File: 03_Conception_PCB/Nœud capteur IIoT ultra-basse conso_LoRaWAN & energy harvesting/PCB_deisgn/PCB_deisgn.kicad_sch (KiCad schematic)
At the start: 24 parts, among them J1 SWD1, U1 AEM10941-QFN, U2 STM32U073C8Ux, Y1 Crystal

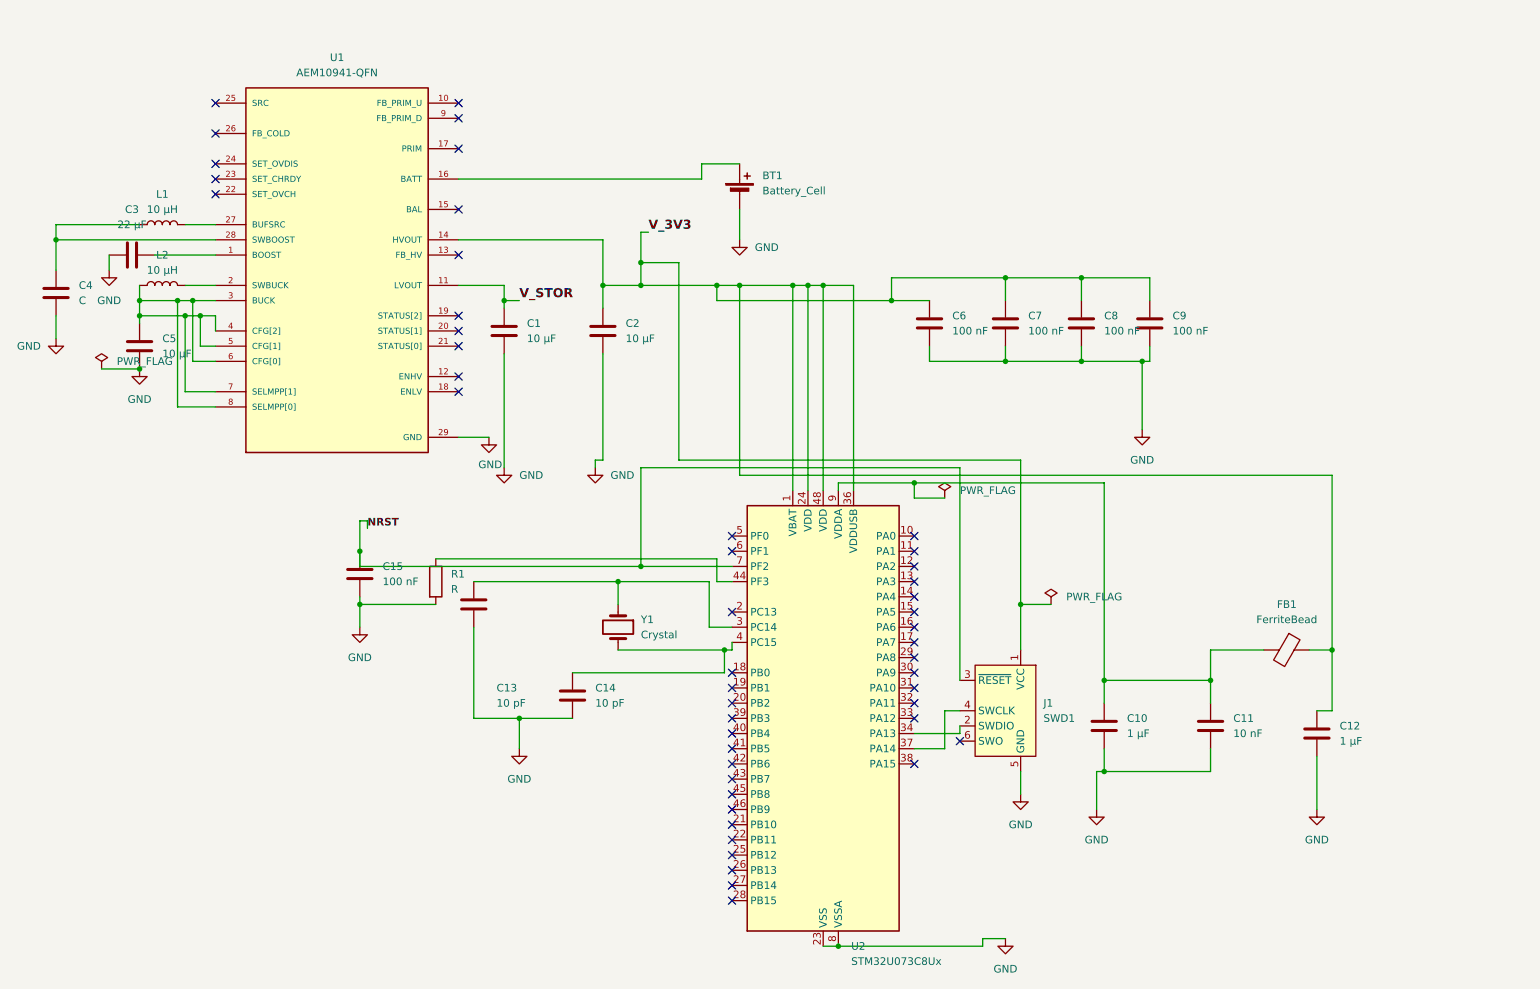
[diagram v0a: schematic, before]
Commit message: UPDATE
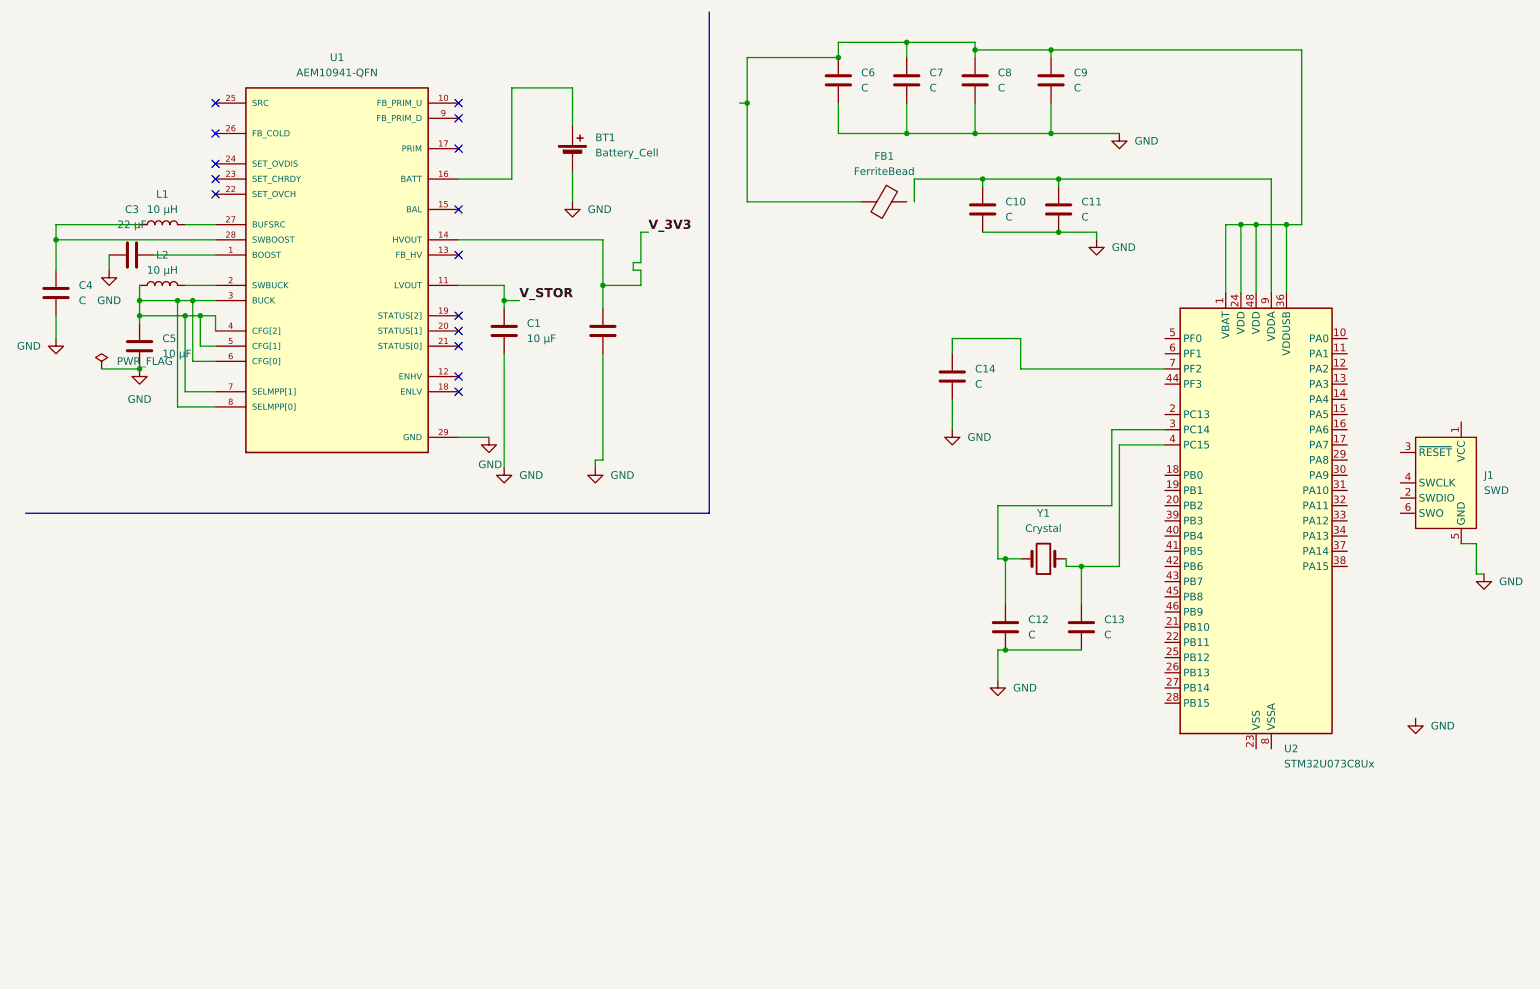
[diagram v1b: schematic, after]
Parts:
- removed C15: 100 nF, symbol Device:C
- removed R1: R, symbol Device:R
- C10, C12: value 1 µF -> C
- C11: value 10 nF -> C
- C13, C14: value 10 pF -> C
- C6, C7, C8, C9: value 100 nF -> C
- FB1: footprint (none) -> Inductor_SMD:L_6.3x6.3_H3
- J1: value SWD1 -> SWD
- Y1: footprint Crystal:Crystal_AT310_D3.0mm_L10.0mm_Horizontal -> (none)
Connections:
- net GND: no longer U2.23 (VSS), U2.35 (VSS), U2.47 (VSS), U2.49 (VSS), U2.8 (VSSA)
- net V_3V3: no longer C12.1, C6.1, C7.1, C8.1, C9.1, FB1.1, J1.1 (VCC), U2.1 (VBAT), U2.24 (VDD), U2.36 (VDDUSB), U2.48 (VDD)
- net at C10.1, C11.1, U2.9 (VDDA): no longer FB1.2
- net at J1.2 (SWDIO): no longer U2.34 (PA13)
- net at J1.4 (SWCLK): no longer U2.37 (PA14)
- net at C13.1, Y1.1: now also U2.4 (PC15); no longer U2.3 (PC14)
- net NRST: no longer names the net of U2.7 (PF2)
- net NRST: now also C14.1; no longer J1.3 (~{RESET})
- new net: C6.1, C7.1, C8.1, C9.1, FB1.2, U2.1 (VBAT), U2.24 (VDD), U2.36 (VDDUSB), U2.48 (VDD)
- new net: C12.1, U2.3 (PC14), Y1.2
- new net: U2.23 (VSS), U2.35 (VSS), U2.47 (VSS), U2.49 (VSS)
- no-connect marks 49 -> 15
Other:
- moved on the sheet: BT1
